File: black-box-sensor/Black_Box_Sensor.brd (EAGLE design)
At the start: 53 x 44 mm, 54 parts, among them J1 104031-0811, J2 UX60-MB-5S8, J3 B4B-PH-SM4-TBT(LF)(SN), U1 ADXL375, U2 ADXL375, U3 ATMEGA32U4-AU, U4 FXAS21002CQR1, U5 MIC5504-3.3YM5-TR, U6 NL27WZ32USG, U7 LT1129CST-5#PBF, U8 AD8426ACPZ-WP, U9 TXU0304

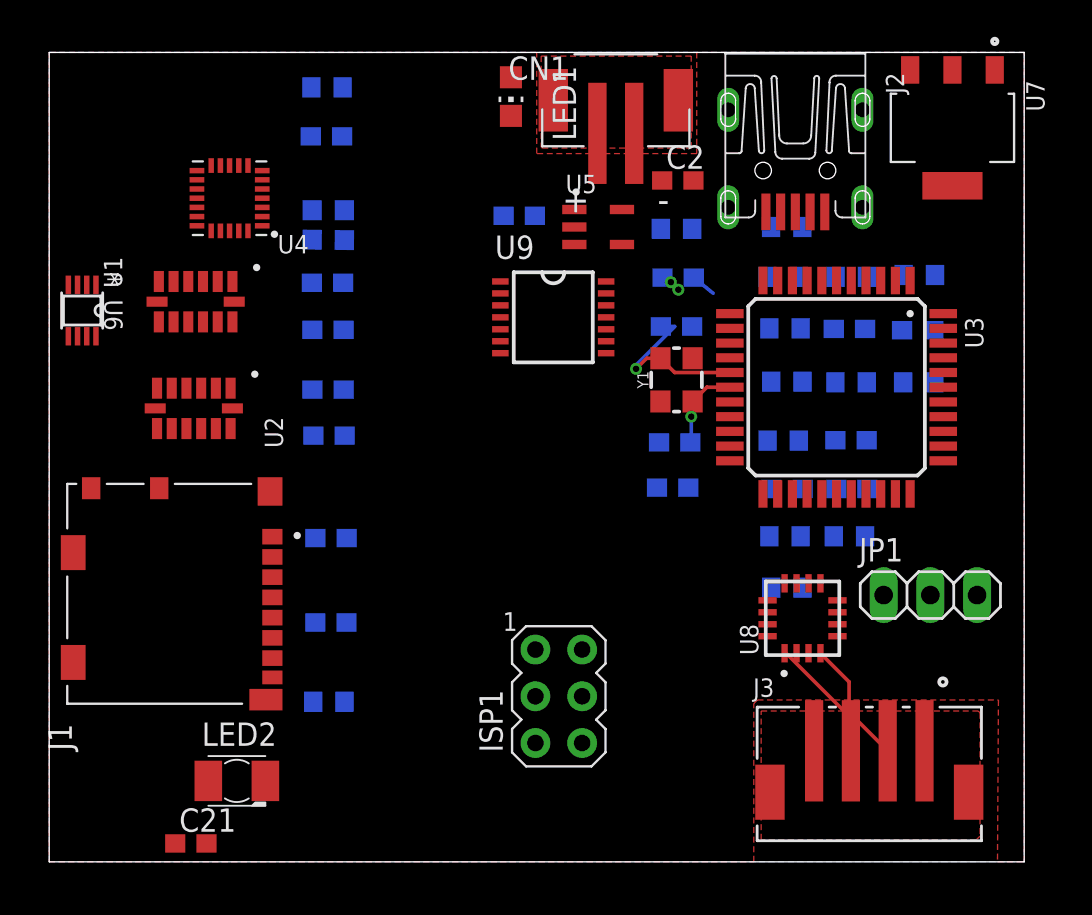
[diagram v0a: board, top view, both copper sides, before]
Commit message: rout
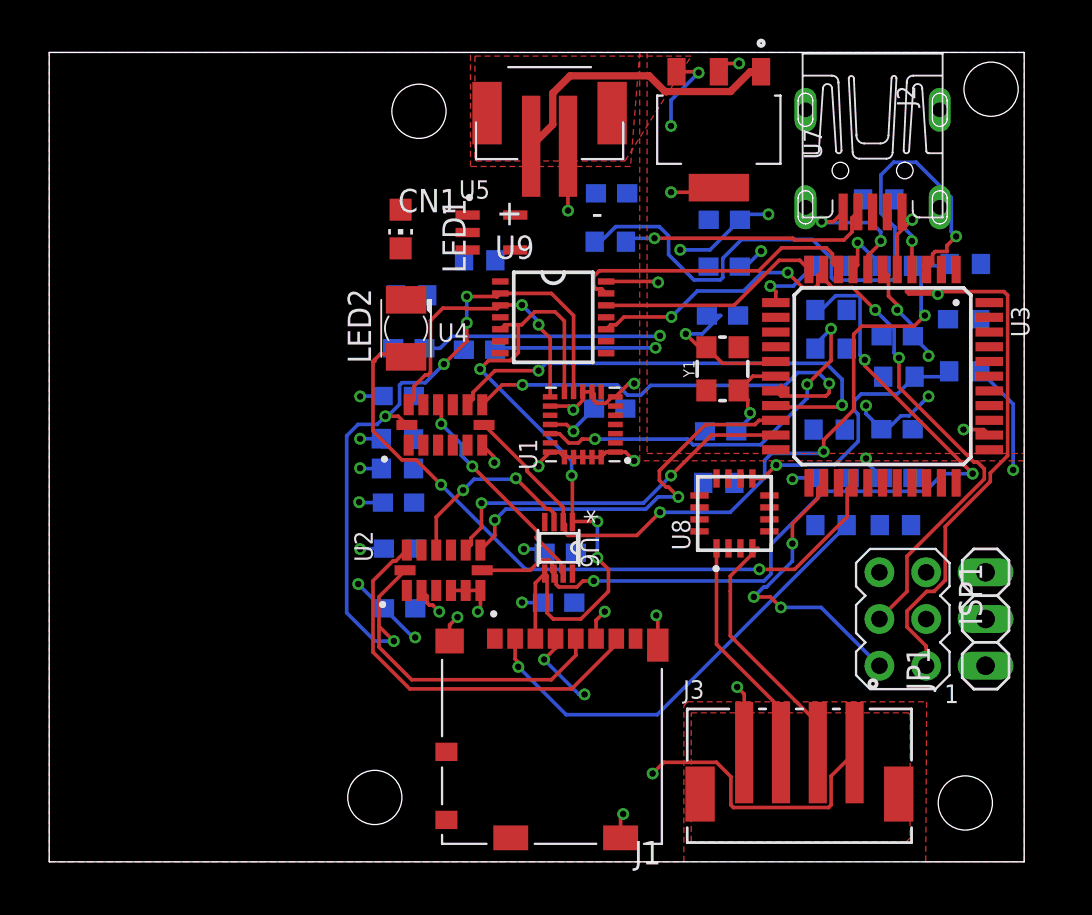
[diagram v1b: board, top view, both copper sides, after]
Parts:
- moved C21 44.6 mm to (36.7, 34.9), flipped to the bottom
- moved U6 28.9 mm to (27.7, 17.1)
- moved LED2 26.3 mm to (19.4, 29.0), turned to 90 degrees
- moved R3 25.4 mm to (23.4, 32.7)
- moved U4 22.8 mm to (29.0, 23.8)
- moved J1 22.1 mm to (27.3, 6.68), turned to 180 degrees
- moved C6 21.4 mm to (30.5, 24.6)
- moved ISP1 19.2 mm to (46.4, 13.2), turned to 180 degrees
- moved U2 16.2 mm to (21.4, 15.8), turned to 90 degrees
- moved C3 15.6 mm to (19.1, 13.8), turned to 180 degrees
- moved U1 15.1 mm to (21.5, 23.8), turned to 90 degrees
- moved C11 14.5 mm to (18.9, 21.4), turned to 180 degrees
- moved C13 12.9 mm to (23.4, 27.8), turned to 0 degrees
- moved U7 12.7 mm to (36.4, 39.8)
- moved C5 12.5 mm to (27.8, 16.8), turned to 180 degrees
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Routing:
- net +5V: track 1.35 -> 63.4 mm, vias 0 -> 15
- net SCLK: track 0.00 -> 55.5 mm, vias 0 -> 5
- net CS2: track 0.00 -> 46.5 mm, vias 0 -> 3
- net MISO_5V: track 0.00 -> 42.7 mm, vias 0 -> 1
- net 3.3V: track 0.00 -> 41.5 mm, vias 0 -> 15
- net CS1: track 0.00 -> 40.6 mm, vias 0 -> 3
- net GND: track 0.64 -> 40.9 mm, vias 2 -> 18
- net MOSI_5V: track 0.00 -> 39.4 mm, vias 0 -> 4
- net MISO: track 0.00 -> 37.9 mm, vias 0 -> 2
- net MOSI: track 0.00 -> 37.8 mm, vias 0 -> 4
- net D-: track 0.00 -> 37.6 mm, vias 0 -> 1
- net LED: track 0.00 -> 37.0 mm, vias 0 -> 2
- net INT1: track 0.00 -> 26.9 mm, vias 0 -> 2
- net CS4: track 0.00 -> 24.8 mm, vias 0 -> 1
- net INT0: track 0.00 -> 24.5 mm, vias 0 -> 2
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- added copper zone on layer 1, net +5V
